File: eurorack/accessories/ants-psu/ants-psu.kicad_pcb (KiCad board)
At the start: 2 copper layers, 70 x 25.9 mm, 17 parts, among them J1 PJ-064B, J2 Conn_02x08_Odd_Even, SW1 SW_SPST

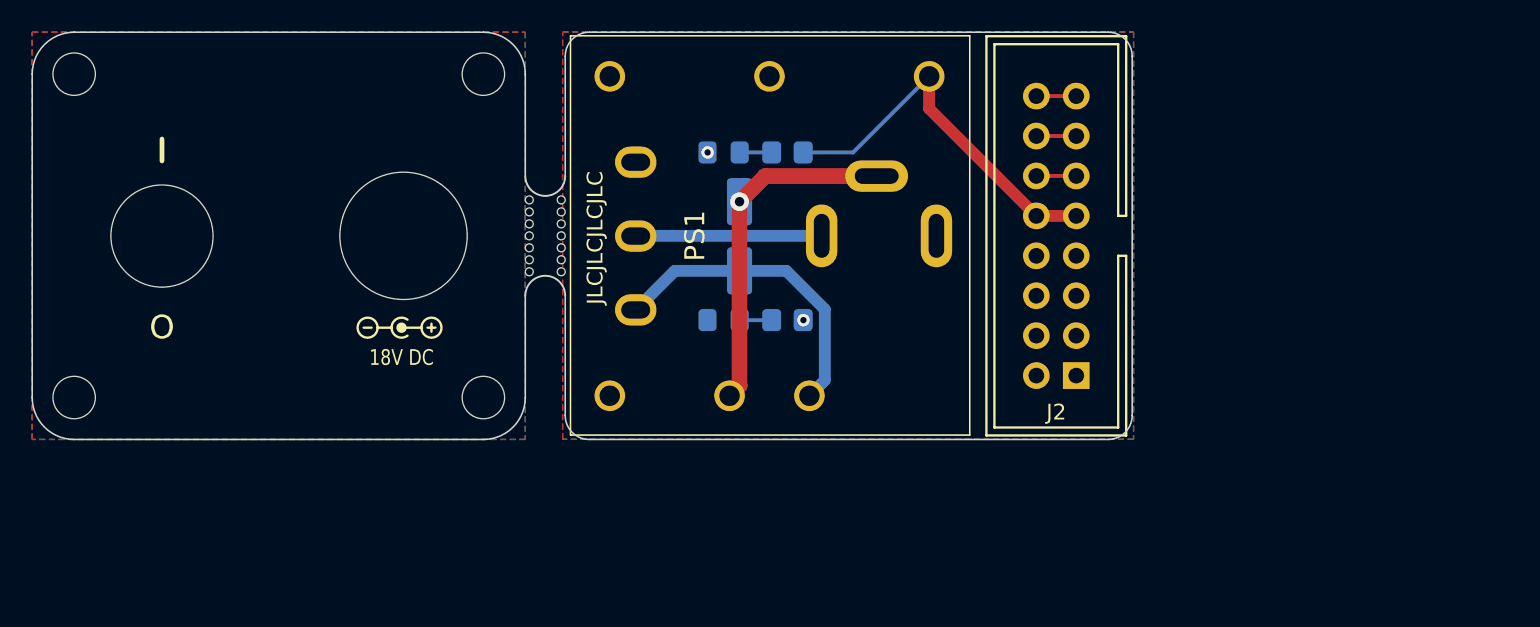
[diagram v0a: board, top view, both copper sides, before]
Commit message: ants v2 final design
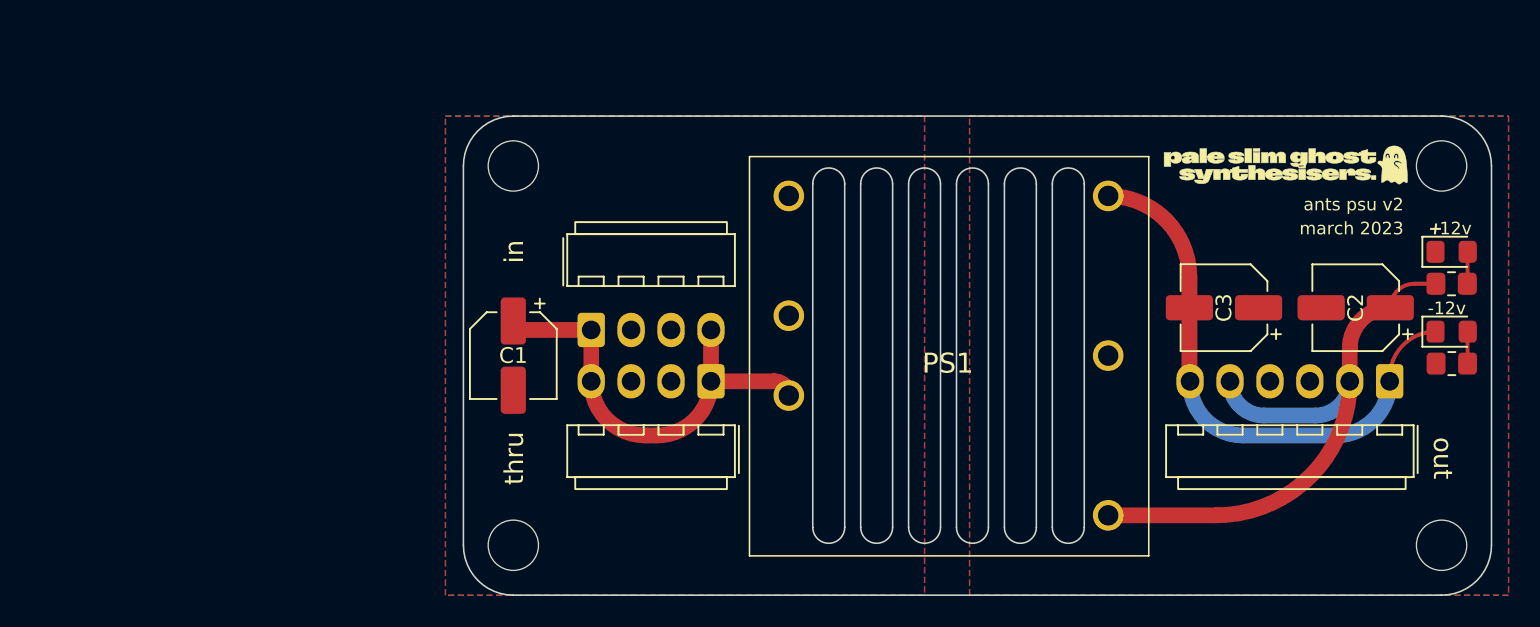
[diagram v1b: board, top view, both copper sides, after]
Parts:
- removed G***: LOGO, LOGO
- removed REF** (x4): MountingHole_2.7mm_M2.5, MountingHole:MountingHole_2.7mm_M2.5
- removed REF** (x2): hole 6mm (jack panel), Pale Slim Ghost:hole 6mm (jack panel)
- removed SW1: SW_SPST, Pale Slim Ghost:Mini Toggle Switch SPDT
- removed mouse-bite-2mm-slot: VAL**, Pale Slim Ghost:mousebite-2.54x5.08mm
- added C2: 47μ, Capacitor_SMD:CP_Elec_5x4.5, F.Cu at (157.0, 92.2)
- added C3: 47μ, Capacitor_SMD:CP_Elec_5x4.5, F.Cu at (148.6, 92.2)
- added H1: MountingHole, MountingHole:MountingHole_3.2mm_M3, F.Cu at (103.4, 83.2)
- added H2: MountingHole, MountingHole:MountingHole_3.2mm_M3, F.Cu at (162.4, 83.2)
- added H3: MountingHole, MountingHole:MountingHole_3.2mm_M3, F.Cu at (162.4, 107.3)
- added H4: MountingHole, MountingHole:MountingHole_3.2mm_M3, F.Cu at (103.4, 107.3)
- added J3: Conn_01x06, Pale Slim Ghost:Molex_KK-254_AE-6410-06A_1x06_P2.54mm_Horizontal, F.Cu at (156.6, 96.9)
- C1, R1, R2: moved to F.Cu
- D1: value LED -> red; moved to F.Cu
- D2: value LED -> blue; moved to F.Cu
- J1: value PJ-064B -> Conn_01x04; footprint Pale Slim Ghost:CUI_PJ-064B -> Pale Slim Ghost:Molex_KK-254_AE-6410-04A_1x04_P2.54mm_Horizontal; moved to F.Cu
- J2: value Conn_02x08_Odd_Even -> Conn_01x04; footprint Pale Slim Ghost:PinHeader_Shrouded_2x08_P2.54mm_Vertical -> Pale Slim Ghost:Molex_KK-254_AE-6410-04A_1x04_P2.54mm_Horizontal
- moved D1 46.7 mm to (163.1, 88.6)
- moved D2 46.3 mm to (163.1, 93.7)
- moved R1 43.1 mm to (163.1, 90.7)
- moved R2 42.4 mm to (163.1, 95.8)
- moved J2 27.2 mm to (112.1, 98.9)
- moved C1 16.3 mm to (103.4, 95.2), turned to -90 degrees
- moved J1 11.6 mm to (112.1, 91.6)
- moved PS1 1.31 mm to (120.9, 97.8), turned to -90 degrees
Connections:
- C1 pad 1: VIN -> VDC
- D1 pad 2: Net-(D1-Pad2) -> Net-(D1-A)
- D2 pad 2: Net-(D2-Pad2) -> Net-(D2-A)
- J1 pad 1: Net-(J1-Pad1) -> VDC
- J1 pad 3: unconnected-(J1-Pad3) -> Earth
- J2 pad 1: -12V -> VDC
- J2 pad 2: -12V -> Earth
- J2 pad 3: GND -> Earth
- J2 pad 4: GND -> VDC
- PS1 pad 1: VIN -> VDC
- R1 pad 1: +12V -> Net-(D1-A)
- R1 pad 2: Net-(D1-Pad2) -> +12V
- R2 pad 1: GND -> Net-(D2-A)
- R2 pad 2: Net-(D2-Pad2) -> GND
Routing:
- net -12V: track 0.00 -> 35.7 mm
- net VDC: track 0.00 -> 28.5 mm
- net Earth: track 22.0 -> 0.00 mm, vias 1 -> 0
- net VIN: track 20.0 -> 0.00 mm
- net +12V: track 24.8 -> 39.6 mm
- net Net-(J1-Pad1): track 11.8 -> 0.00 mm
- net Gate: track 2.54 -> 0.00 mm
- net CV: track 2.54 -> 0.00 mm
- net +5V: track 2.54 -> 0.00 mm
- net Net-(D1-A): track 0.00 -> 2.05 mm
- net Net-(D2-Pad2): track 2.04 -> 0.00 mm
- net Net-(D1-Pad2): track 2.04 -> 0.00 mm
- net Net-(D2-A): track 0.00 -> 2.04 mm
- net GND: vias 2 -> 0
- added copper zone on B.Cu, net Earth
- added copper zone on F.Cu, net Earth
- added copper zone on B.Cu, net GND
- removed copper zone on B.Cu, net (none)
- removed copper zone on F.Cu, net (none)
- removed copper zone on B.Cu, net -12V
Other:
- board size 70 x 25.9 mm -> 65.4 x 30.5 mm
- board text added: "+"
- board text added: "-12v"
- board text added: "12v"
- board text added: "ants psu v2"
- board text added: "in"
- board text added: "march 2023"
- board text added: "out"
- board text added: "thru"
- board text removed: "18V DC"
- board text removed: "Ants v1 ∙ December 2021"
- board text removed: "JLCJLCJLCJLC"
- board text removed: "O"
